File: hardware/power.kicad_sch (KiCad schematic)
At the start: 17 parts, among them Q2 SI2347DS-T1-GE3, U7 NCP565D2T33R4G, U8 SI06W8-05

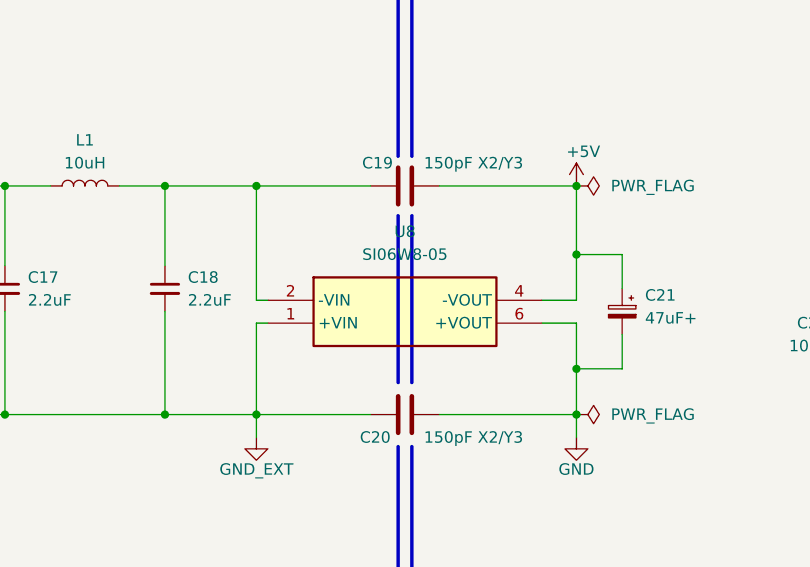
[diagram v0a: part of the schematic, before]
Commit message: Finished pcb routing
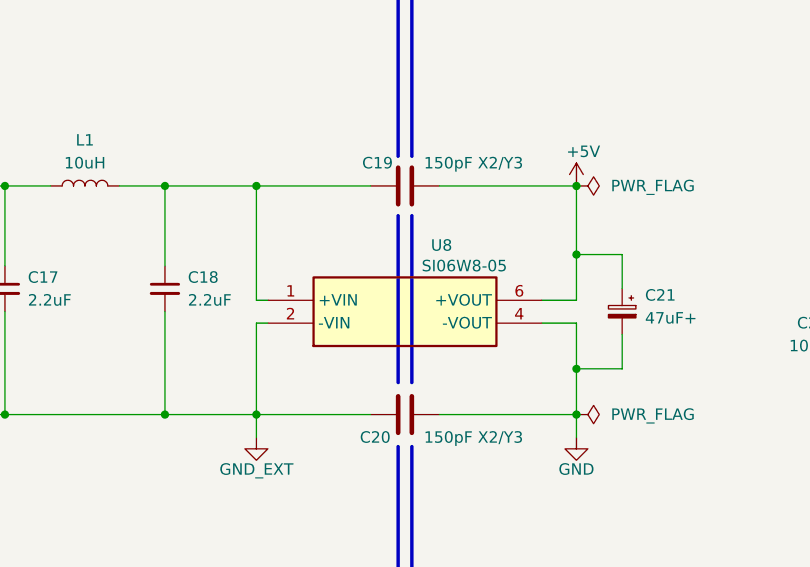
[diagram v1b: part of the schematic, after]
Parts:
- U8: Mouser Part Number https://www.mouser.pl/ProductDetail/MEAN-WELL/SI06W8-05?qs=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 -> (none)
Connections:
- net +5V: now also U8.6 (+VOUT); no longer U8.4 (-VOUT)
- net GND: now also U8.4 (-VOUT); no longer U8.6 (+VOUT)
- net GND_EXT: now also U8.2 (-VIN); no longer U8.1 (+VIN)
- net at C18.1, C19.1, L1.2: now also U8.1 (+VIN); no longer U8.2 (-VIN)
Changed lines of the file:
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@@
 	(wire
 		(pts
+			(xy 165.1 95.25) (xy 168.91 95.25)
+		)
+		(stroke
+			(width 0)
+			(type default)
+		)
+	)
+	(wire
+		(pts
 			(xy 168.91 97.79) (xy 168.91 102.87)
 		)
@@
 	(wire
 		(pts
-			(xy 133.35 95.25) (xy 134.62 95.25)
-		)
-		(stroke
-			(width 0)
-			(type default)
-		)
-	)
-	(wire
-		(pts
 			(xy 123.19 107.95) (xy 133.35 107.95)
 		)
@@
 	(wire
 		(pts
+			(xy 133.35 95.25) (xy 134.62 95.25)
+		)
+		(stroke
+			(width 0)
+			(type default)
+		)
+	)
+	(wire
+		(pts
 			(xy 200.66 93.98) (xy 200.66 95.25)
 		)
@@
 	(wire
 		(pts
-			(xy 165.1 95.25) (xy 168.91 95.25)
-		)
-		(stroke
-			(width 0)
-			(type default)
-		)
-	)
-	(wire
-		(pts
 			(xy 134.62 97.79) (xy 133.35 97.79)
 		)
@@
 	(symbol
 		(lib_id "SI06W8-05:SI06W8-05")
-		(at 134.62 95.25 0)
+		(at 134.62 97.79 0)
+		(mirror x)
 		(unit 1)
 		(body_style 1)
@@
 		(in_pos_files yes)
 		(dnp no)
-		(fields_autoplaced yes)
 		(property "Reference" "U8"
-			(at 149.86 87.63 0)
+			(at 153.924 89.154 0)
 			(show_name no)
 			(do_not_autoplace no)
@@
 		)
 		(property "Value" "SI06W8-05"
-			(at 149.86 90.17 0)
+			(at 156.464 91.44 0)
 			(show_name no)
 			(do_not_autoplace no)
@@
 		)
 		(property "Footprint" "DCisoconv:SI06W805"
-			(at 161.29 190.17 0)
+			(at 161.29 2.87 0)
 			(hide yes)
 			(show_name no)
@@
 		)
 		(property "Datasheet" "https://www.meanwell.com/upload/pdf/DI06W8/SI06W8,DI06W8-spec.pdf"
-			(at 161.29 290.17 0)
+			(at 161.29 -97.13 0)
 			(hide yes)
 			(show_name no)
@@
 		)
 		(property "Description" "Isolated DC/DC Converters - Through Hole 6W 9-75Vin 5V 0-1200mA 1x1 Regulated DIP"
-			(at 134.62 95.25 0)
-			(hide yes)
-			(show_name no)
-			(do_not_autoplace no)
-			(effects
-				(font
-					(size 1.27 1.27)
-				)
-			)
-		)
-		(property "Mouser Part Number" "https://www.mouser.pl/ProductDetail/MEAN-WELL/SI06W8-05?qs=ST9lo4GX8V3OoQwDIibogw%3D%3D"
-			(at 161.29 590.17 0)
-			(hide yes)
-			(show_name no)
-			(do_not_autoplace no)
-			(effects
-				(font
-					(size 1.27 1.27)
-				)
-				(justify left top)
-			)
-		)
-		(property "Author" ""
-			(at 134.62 95.25 0)
-			(hide yes)
-			(show_name no)
-			(do_not_autoplace no)
-			(effects
-				(font
-					(size 1.27 1.27)
-				)
-			)
-		)
-		(property "License" ""
-			(at 134.62 95.25 0)
-			(hide yes)
-			(show_name no)
-			(do_not_autoplace no)
-			(effects
-				(font
-					(size 1.27 1.27)
-				)
-			)
-		)
-		(property "MPN" ""
-			(at 134.62 95.25 0)
-			(hide yes)
-			(show_name no)
-			(do_not_autoplace no)
-			(effects
-				(font
-					(size 1.27 1.27)
-				)
-			)
-		)
-		(property "Manufacturer" ""
-			(at 134.62 95.25 0)
+			(at 134.62 97.79 0)
 			(hide yes)
 			(show_name no)
@@
 		)
 		(property "Mouser" "https://www.mouser.pl/ProductDetail/MEAN-WELL/SI06W8-05?qs=ST9lo4GX8V3OoQwDIibogw%3D%3D"
-			(at 134.62 95.25 0)
-			(hide yes)
-			(show_name no)
-			(do_not_autoplace no)
-			(effects
-				(font
-					(size 1.27 1.27)
-				)
-			)
-		)
-		(property "Sim.Device" ""
-			(at 134.62 95.25 0)
-			(hide yes)
-			(show_name no)
-			(do_not_autoplace no)
-			(effects
-				(font
-					(size 1.27 1.27)
-				)
-			)
-		)
-		(property "Sim.Type" ""
-			(at 134.62 95.25 0)
+			(at 134.62 97.79 0)
 			(hide yes)
 			(show_name no)
